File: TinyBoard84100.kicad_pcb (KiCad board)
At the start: 2 copper layers, 25.7 x 15.2 mm, 13 parts, among them P2 CONN_01X07, P3 CONN_01X07, P4 CONN_02X03, SW1 SW_PUSH, U1 78L05, U2 ATTINY841

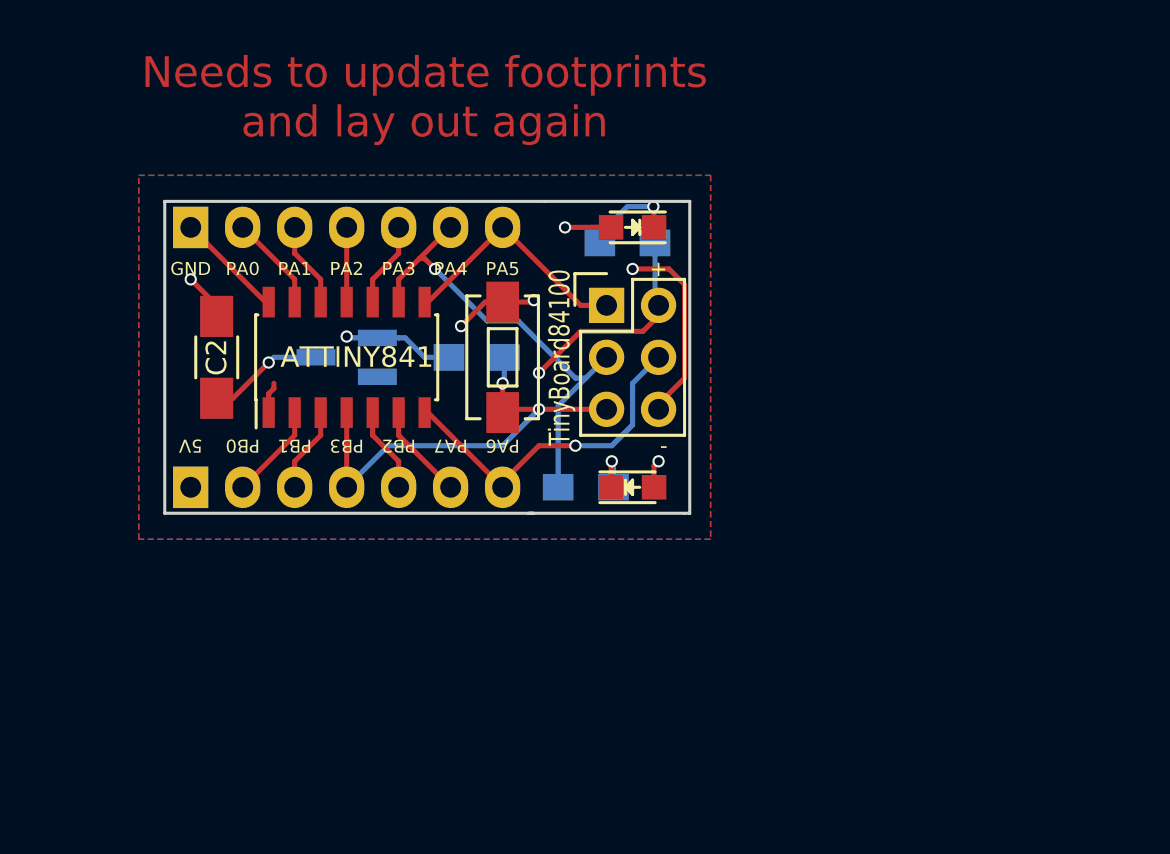
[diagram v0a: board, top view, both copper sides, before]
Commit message: starting over
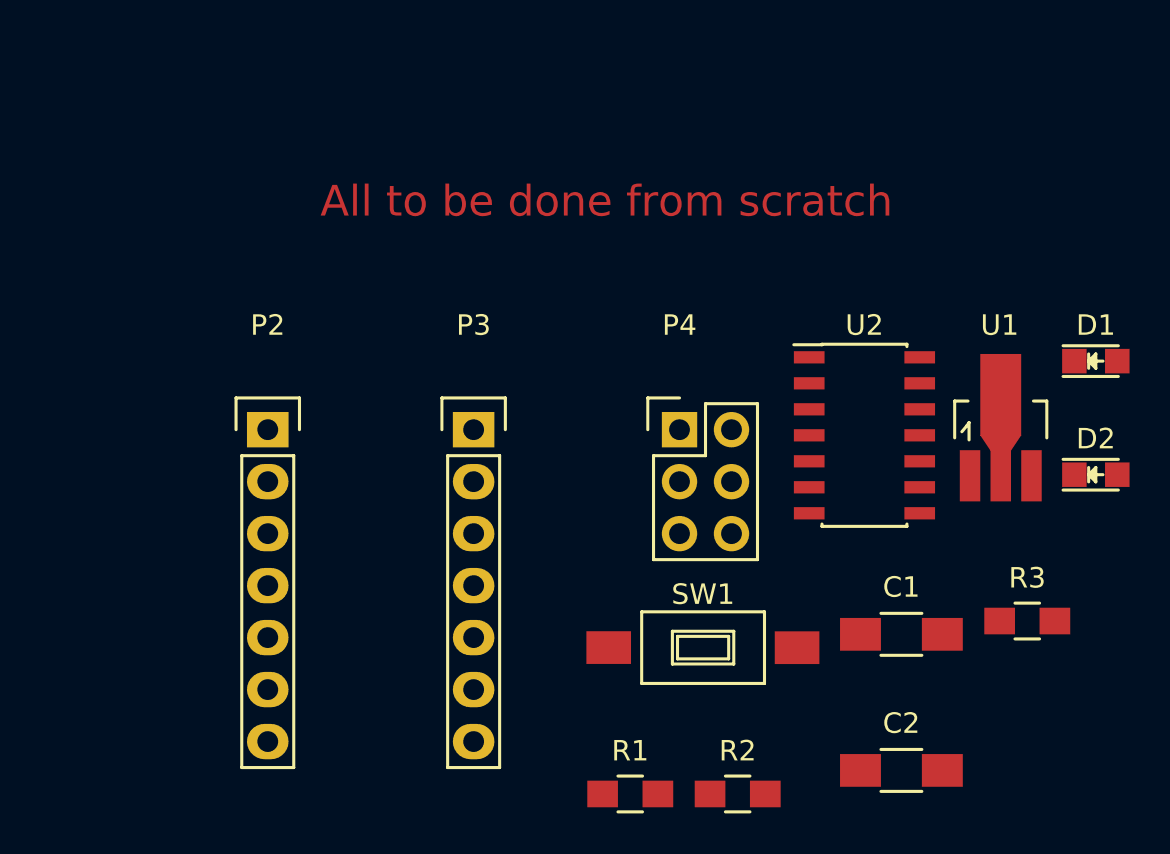
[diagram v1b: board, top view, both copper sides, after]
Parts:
- C1, P2, P3, R1, R2, R3: moved to F.Cu
- SW1: footprint Buttons_Switches_SMD:SW_SPST_EVQPE1 -> Buttons_Switches_SMD:SW_SPST_FSMSM
- U1: footprint TO_SOT_Packages_SMD:SOT-23_Handsoldering -> TO_SOT_Packages_SMD:SOT89-3_Housing_Handsoldering; moved to F.Cu
- moved C2 39.1 mm to (192.2, 100.2), turned to 0 degrees
- moved C1 36.1 mm to (192.2, 93.5), turned to 0 degrees
- moved U1 32.1 mm to (197.1, 83.4), turned to 0 degrees
- moved R2 27.5 mm to (184.2, 101.3), turned to 0 degrees
- moved U2 25.6 mm to (190.4, 83.8), turned to 0 degrees
- moved D1 23.6 mm to (201.7, 80.2), turned to 0 degrees
- moved D2 22.6 mm to (201.7, 85.7)
- moved R1 22.6 mm to (179.0, 101.3)
- moved R3 22.5 mm to (198.4, 92.9)
- moved SW1 17.2 mm to (182.5, 94.2), turned to 0 degrees
- moved P3 17.0 mm to (171.3, 83.5), turned to 0 degrees
- moved P4 7.04 mm to (181.4, 83.5)
- moved P2 4.70 mm to (161.2, 83.5), turned to 0 degrees
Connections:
- C1 pad 1: Net-(C1-Pad1) -> +BATT
- C2 pad 1: Net-(C1-Pad1) -> +BATT
- P2 pad 1: +5V -> +BATT
- U1 pad 3: Net-(C1-Pad1) -> +BATT
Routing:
- net GND: track 25.8 -> 0.00 mm, vias 6 -> 0
- net /PA4: track 22.6 -> 0.00 mm, vias 1 -> 0
- net /PB3: track 22.5 -> 0.00 mm, vias 2 -> 0
- net +5V: track 17.7 -> 0.00 mm, vias 2 -> 0
- net /PA6: track 16.9 -> 0.00 mm, vias 1 -> 0
- net /PA5: track 12.0 -> 0.00 mm
- net Net-(C1-Pad1): track 5.68 -> 0.00 mm, vias 1 -> 0
- net /PA7: track 4.70 -> 0.00 mm
- net /PB0: track 4.70 -> 0.00 mm
- net /PA0: track 4.70 -> 0.00 mm
- net Net-(D1-Pad1): track 4.64 -> 0.00 mm, vias 1 -> 0
- net /PA1: track 4.18 -> 0.00 mm
- net /PB1: track 4.18 -> 0.00 mm
- net /PA3: track 4.18 -> 0.00 mm
- net /PB2: track 4.18 -> 0.00 mm
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- removed copper zone on F.Cu, net +5V
- removed copper zone on B.Cu, net GND
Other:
- board outline removed
- board text added: "All to be done from scratch"
- board text removed: "+"
- board text removed: "-"
- board text removed: "04/18"
- board text removed: "5V"
- board text removed: "GND"
- board text removed: "Needs to update footprints and lay out again"
- board text removed: "PA0"
- board text removed: "PA1"
- board text removed: "PA2"
- board text removed: "PA3"
- board text removed: "PA4"
- board text removed: "PA5"
- board text removed: "PA6"
- board text removed: "PA7"
- board text removed: "PB0"
- board text removed: "PB1"
- board text removed: "PB2"
- board text removed: "PB3"
- board text removed: "Rev2"
- board text removed: "TinyBoard84100"
- board text removed: "Unregulated Powersupply"
